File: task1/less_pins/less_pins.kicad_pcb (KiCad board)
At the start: 2 copper layers, 27 x 20 mm, 14 parts, among them IC1 NPM1100-QDAA-R7, J1 USB_B_Micro, J2 Power Header, J3 Battery Header

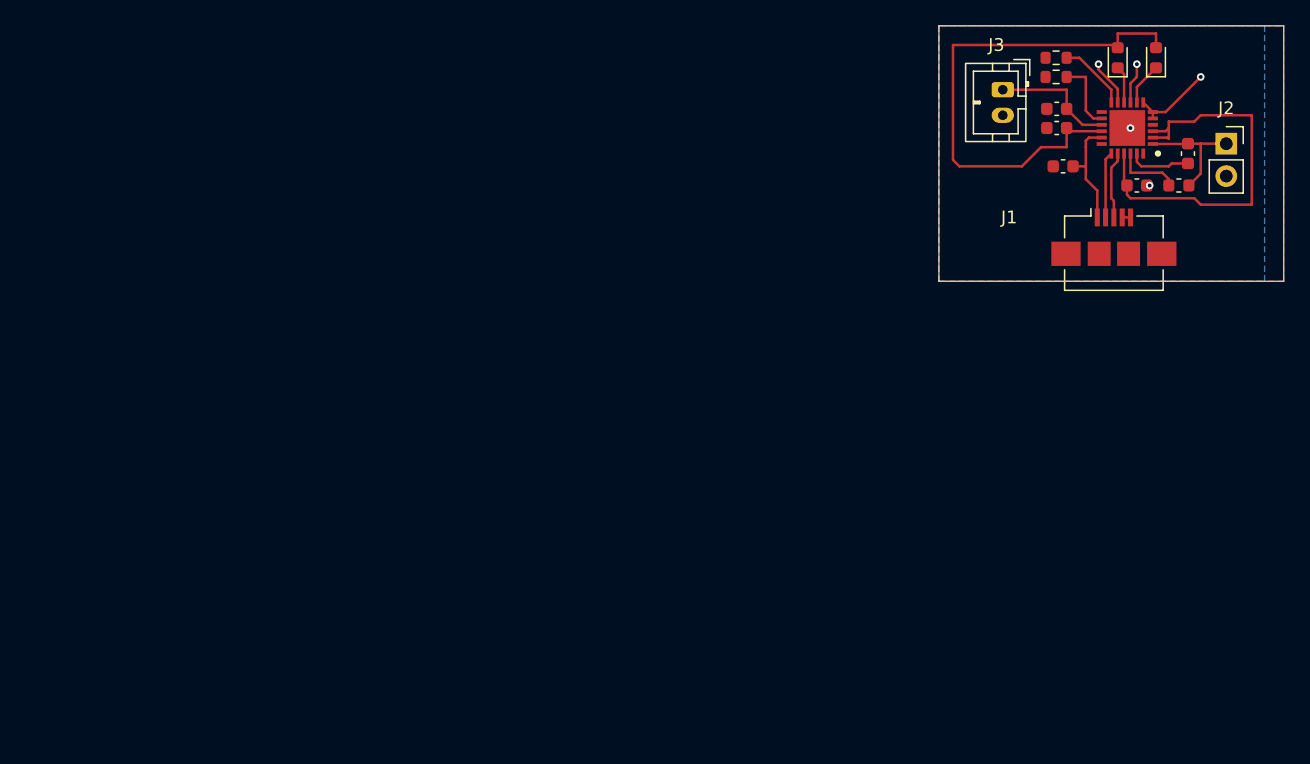
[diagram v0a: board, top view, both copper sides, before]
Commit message: added a new build
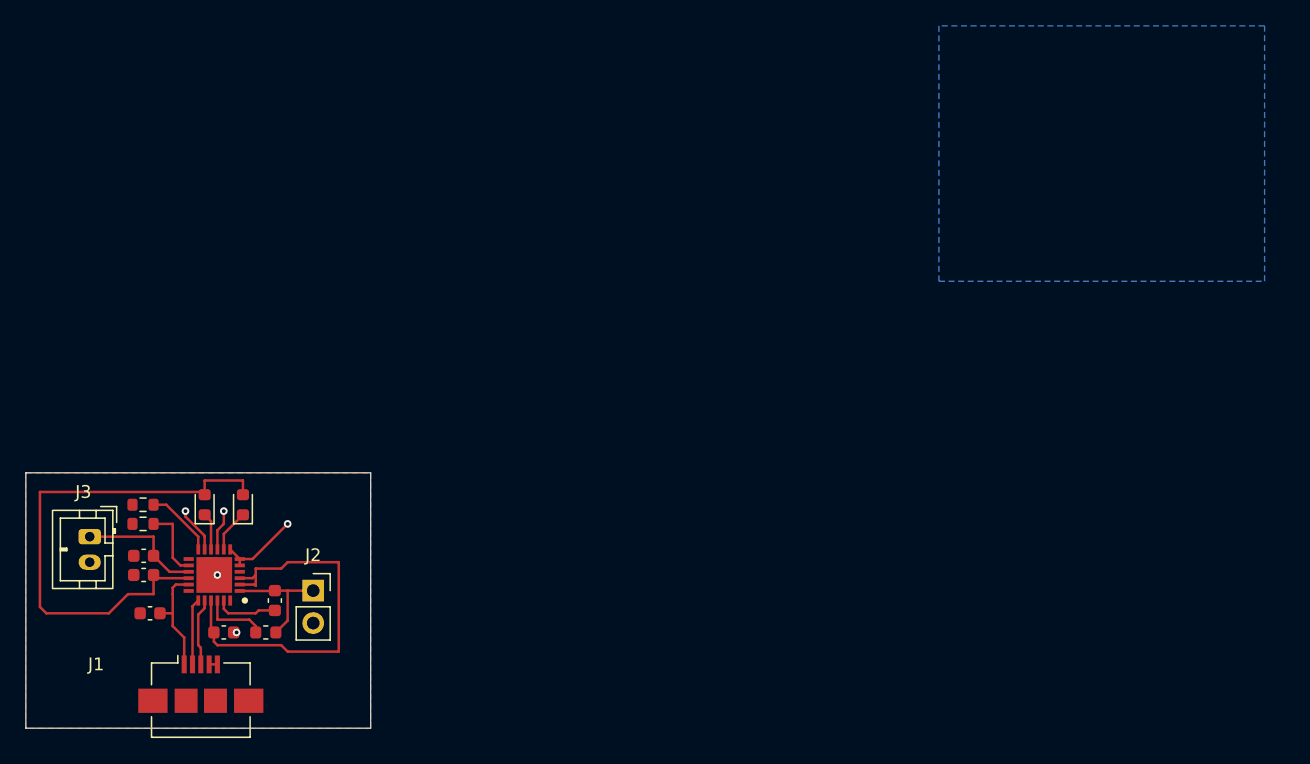
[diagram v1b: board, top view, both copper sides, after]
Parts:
- moved C1 79.6 mm to (152.0, 103.0)
- moved C2 79.6 mm to (141.7, 99.5)
- moved C3 79.6 mm to (148.0, 105.5)
- moved C4 79.6 mm to (142.2, 104.0)
- moved C5 79.6 mm to (141.7, 101.0)
- moved D1 79.6 mm to (149.5, 95.5)
- moved D2 79.6 mm to (146.5, 95.5)
- moved IC1 79.6 mm to (147.2, 101.0)
- moved J1 79.6 mm to (146.2, 109.5)
- moved J2 79.6 mm to (155.0, 102.2)
- moved J3 79.6 mm to (137.5, 98.0)
- moved L1 79.6 mm to (151.3, 105.5)
- moved R1 79.6 mm to (141.7, 97.0)
- moved R2 79.6 mm to (141.7, 95.5)
